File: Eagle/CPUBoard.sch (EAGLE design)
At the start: 33 parts, among them IC2 MAX232, IC3 MAX485CPA, J1 DISPLAY, J2 BUTTON_BOARD, J3 RELAY_BOARD, Q1 12.000MHz, X6 MKDSN1,5/3-5,08, X7 MKDSN1,5/3-5,08

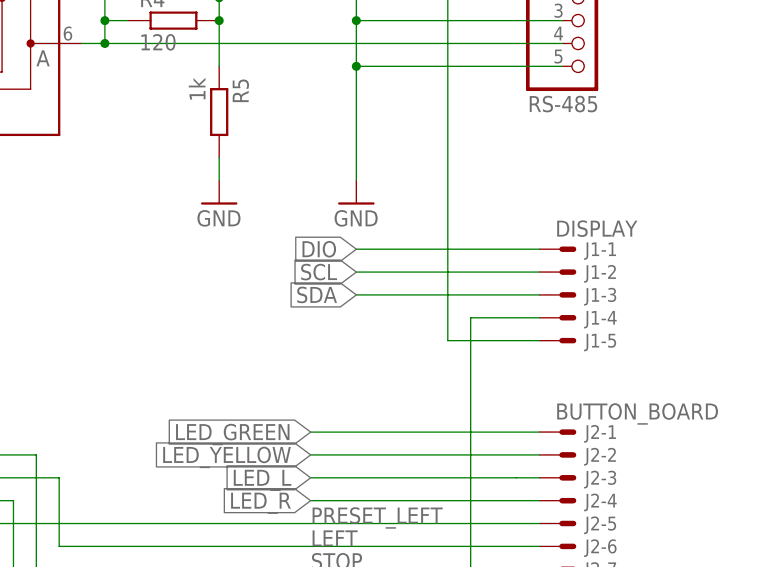
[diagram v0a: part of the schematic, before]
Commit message: - another fix for the TWI pins, hopefully the last one!
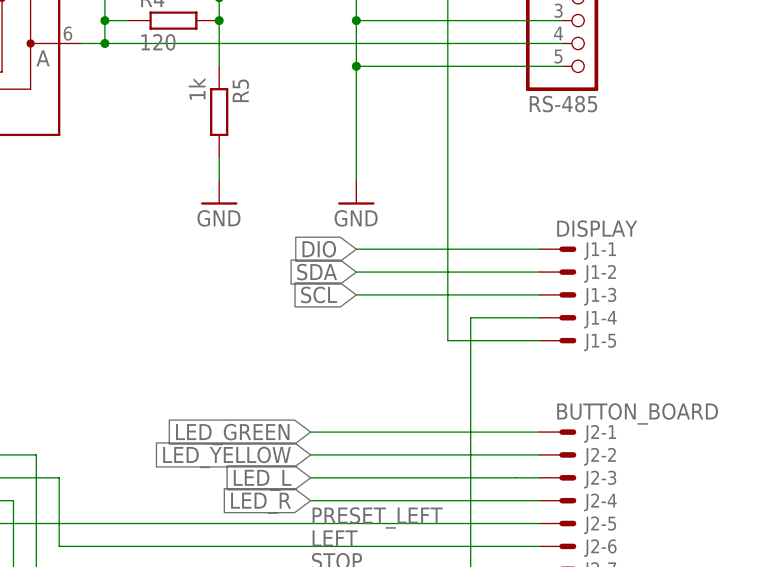
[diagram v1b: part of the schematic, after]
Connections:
- net SCL: now also J1-3.S; no longer J1-2.S
- net SDA: now also J1-2.S; no longer J1-3.S
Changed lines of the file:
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@@
 </segment>
 <segment>
-<label x="220.98" y="121.92" size="1.778" layer="95" rot="MR0" xref="yes"/>
-<wire x1="241.3" y1="121.92" x2="220.98" y2="121.92" width="0.1524" layer="91"/>
-<pinref part="J1" gate="-2" pin="S"/>
+<label x="220.98" y="119.38" size="1.778" layer="95" rot="MR0" xref="yes"/>
+<wire x1="241.3" y1="119.38" x2="220.98" y2="119.38" width="0.1524" layer="91"/>
+<pinref part="J1" gate="-3" pin="S"/>
 </segment>
 </net>
@@
 </segment>
 <segment>
-<label x="220.98" y="119.38" size="1.778" layer="95" rot="MR0" xref="yes"/>
-<wire x1="241.3" y1="119.38" x2="220.98" y2="119.38" width="0.1524" layer="91"/>
-<pinref part="J1" gate="-3" pin="S"/>
+<label x="220.98" y="121.92" size="1.778" layer="95" rot="MR0" xref="yes"/>
+<pinref part="J1" gate="-2" pin="S"/>
+<wire x1="220.98" y1="121.92" x2="241.3" y2="121.92" width="0.1524" layer="91"/>
 </segment>
 </net>
